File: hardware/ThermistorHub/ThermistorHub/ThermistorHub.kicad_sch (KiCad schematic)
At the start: 0 parts

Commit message: 一旦
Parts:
- added A101: ~, Library:XIAO-ESP32S3-DIP, symbol New_Library_0:xiao_ESP32S3
- added J101: Battery, symbol Connector_Generic:Conn_01x02
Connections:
- new net: A101.15 (BAT+), J101.2 (Pin_2)
- new net: A101.16 (BAT-), J101.1 (Pin_1)
- new net GND: A101.13 (GND)
- new net Thermistor/R_Thermistor1: A101.1 (GPIO1)
- new net Thermistor/R_Thermistor2: A101.2 (GPIO2)
- new net Thermistor/R_Thermistor3: A101.3 (GPIO3)
- new net Thermistor/R_Thermistor4: A101.4 (GPIO4)
- new net Thermistor/R_Thermistor5: A101.5 (GPIO5)
- new net Thermistor/R_Thermistor6: A101.6 (GPIO6)
- new net VDD: A101.12 (3V3)
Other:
- added sheet SD (untitled.kicad_sch)
- added sheet Thermistor (Thermistor.kicad_sch)

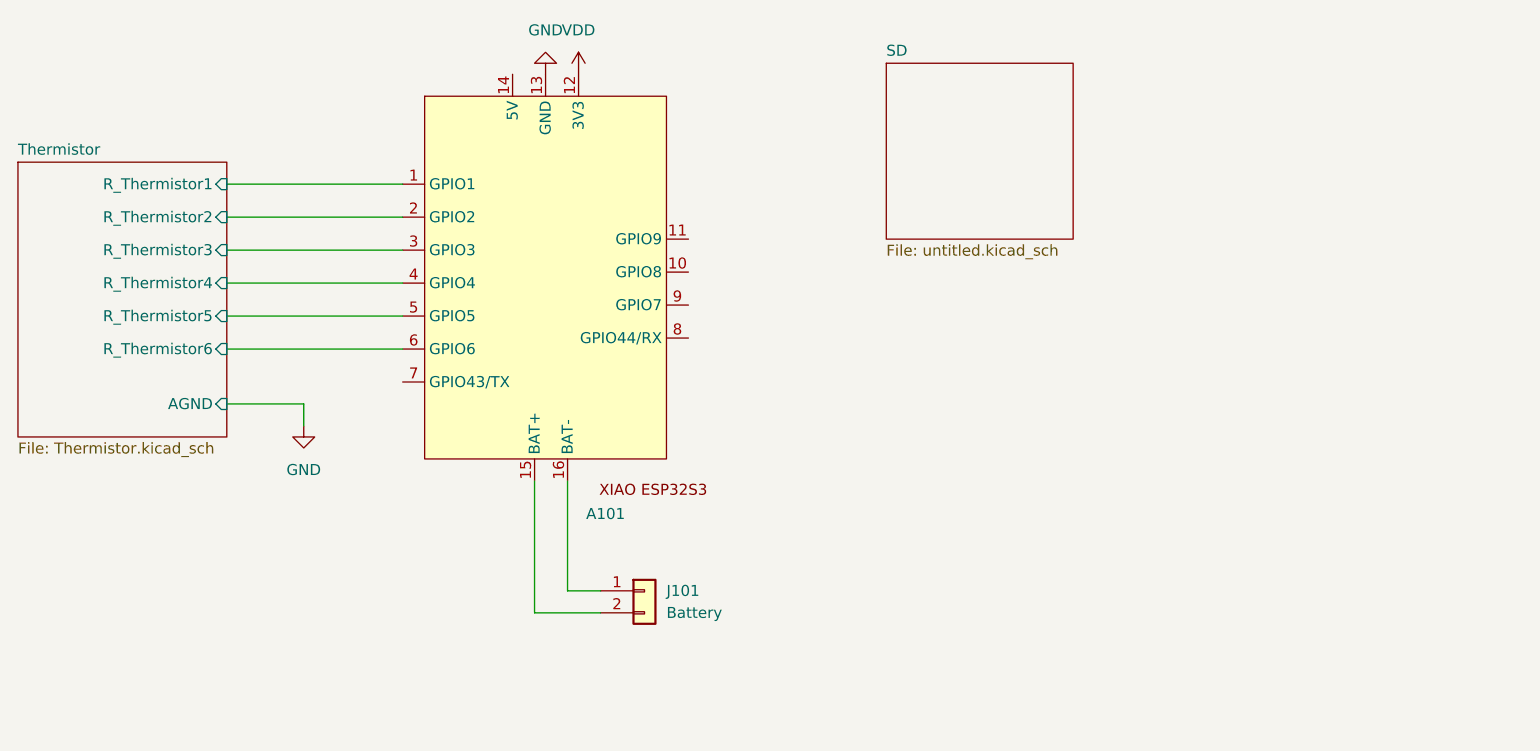
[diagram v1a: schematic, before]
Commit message: 発注
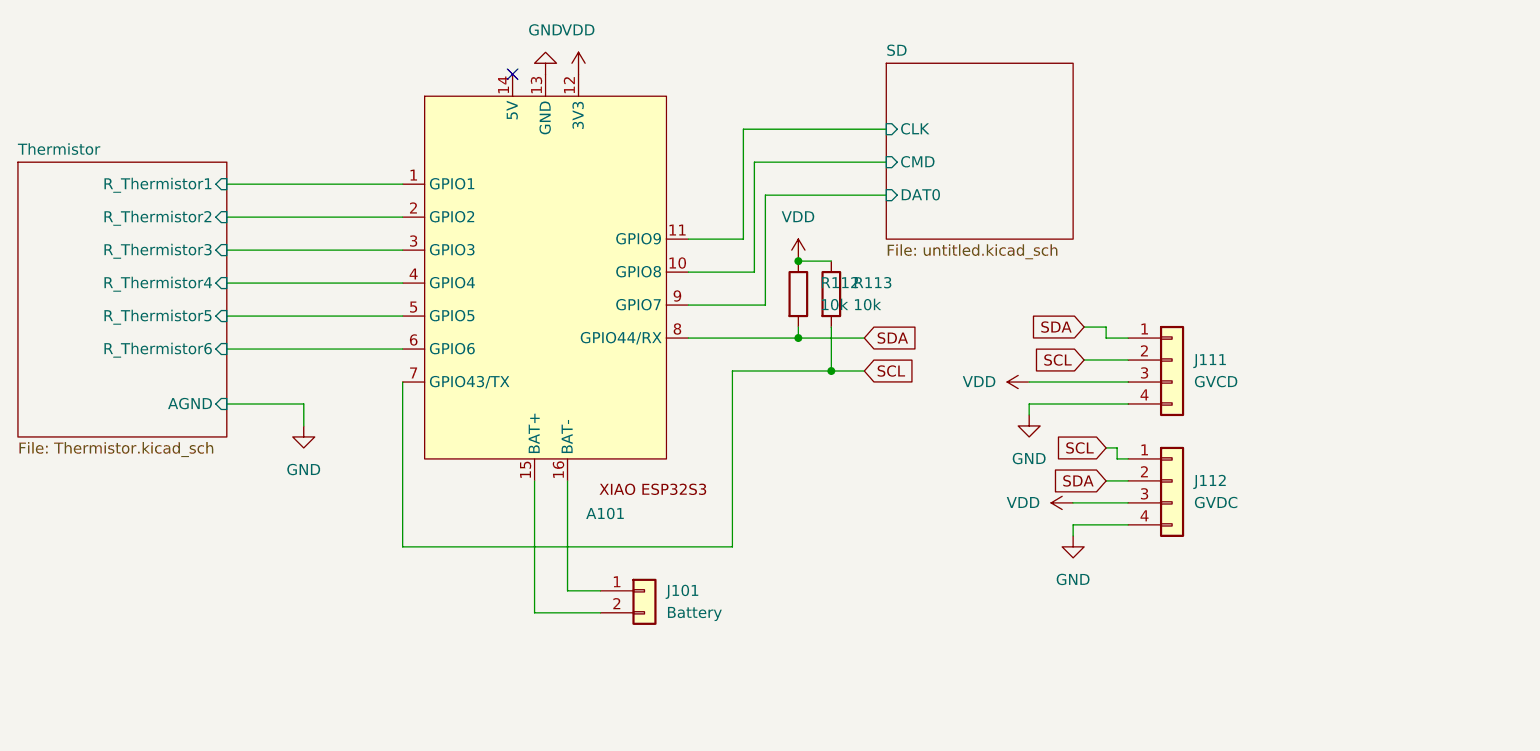
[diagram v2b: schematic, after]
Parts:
- added J111: GVCD, Connector_PinHeader_2.54mm:PinHeader_1x04_P2.54mm_Vertical, symbol Connector_Generic:Conn_01x04
- added J112: GVDC, Connector_PinHeader_2.54mm:PinHeader_1x04_P2.54mm_Vertical, symbol Connector_Generic:Conn_01x04
- added R112, R113: 10k, Resistor_THT:R_Axial_DIN0204_L3.6mm_D1.6mm_P5.08mm_Horizontal, symbol Device:R
- J101: footprint (none) -> Connector_JST:JST_PH_B2B-PH-K_1x02_P2.00mm_Vertical
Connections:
- net GND: now also J111.4 (Pin_4), J112.4 (Pin_4)
- net VDD: now also J111.3 (Pin_3), J112.3 (Pin_3), R112.1, R113.1
- net SD/CMD: now reaches A101.10 (GPIO8)
- net SD/CLK: now reaches A101.11 (GPIO9)
- net SCL: now reaches A101.7 (GPIO43/TX)
- net SCL: now also J111.2 (Pin_2), J112.1 (Pin_1), R113.2
- net SDA: now reaches A101.8 (GPIO44/RX)
- net SDA: now also J111.1 (Pin_1), J112.2 (Pin_2), R112.2
- net SD/DAT0: now reaches A101.9 (GPIO7)
- no-connect marks 0 -> 1
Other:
- sheet SD ports: added CLK, CMD, DAT0; removed none

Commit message: 諸々
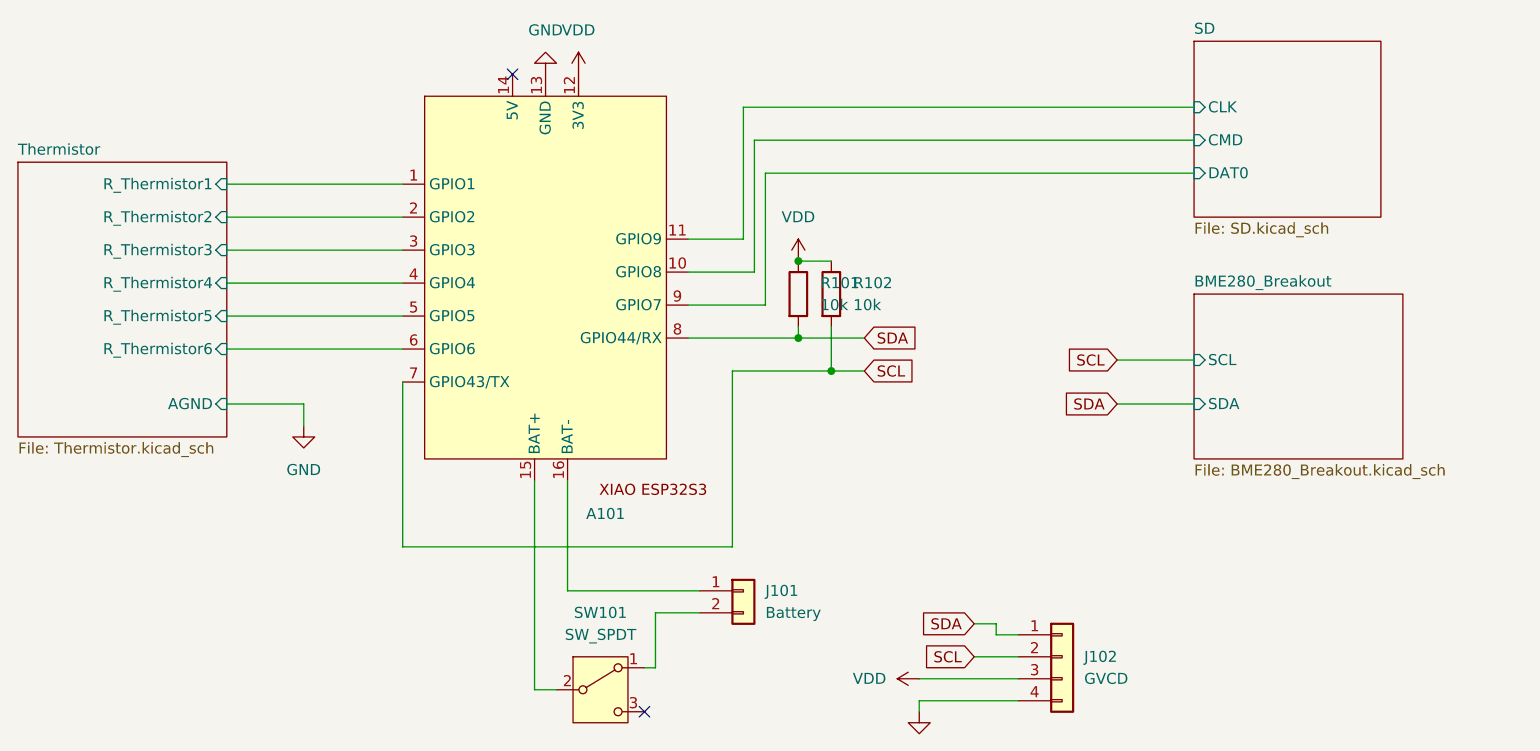
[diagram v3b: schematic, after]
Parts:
- removed J112: GVDC, Connector_PinHeader_2.54mm:PinHeader_1x04_P2.54mm_Vertical, symbol Connector_Generic:Conn_01x04
- added SW101: SW_SPDT, Button_Switch_THT:SW_Slide-03_Wuerth-WS-SLTV_10x2.5x6.4_P2.54mm, symbol Switch:SW_SPDT
- renumbered J111 to J102, R112 to R101, R113 to R102
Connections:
- net at J101.2 (Pin_2): now also SW101.1 (A); no longer A101.15 (BAT+)
- new net: A101.15 (BAT+), SW101.2 (B)
- no-connect marks 1 -> 2
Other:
- added sheet BME280_Breakout (BME280_Breakout.kicad_sch)
- sheet SD: file untitled.kicad_sch -> SD.kicad_sch
- moved on the sheet: J101, J102
